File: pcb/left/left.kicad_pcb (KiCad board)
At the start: 2 copper layers, 27.9 x 72.4 mm, 21 parts, among them J1 Conn_01x07

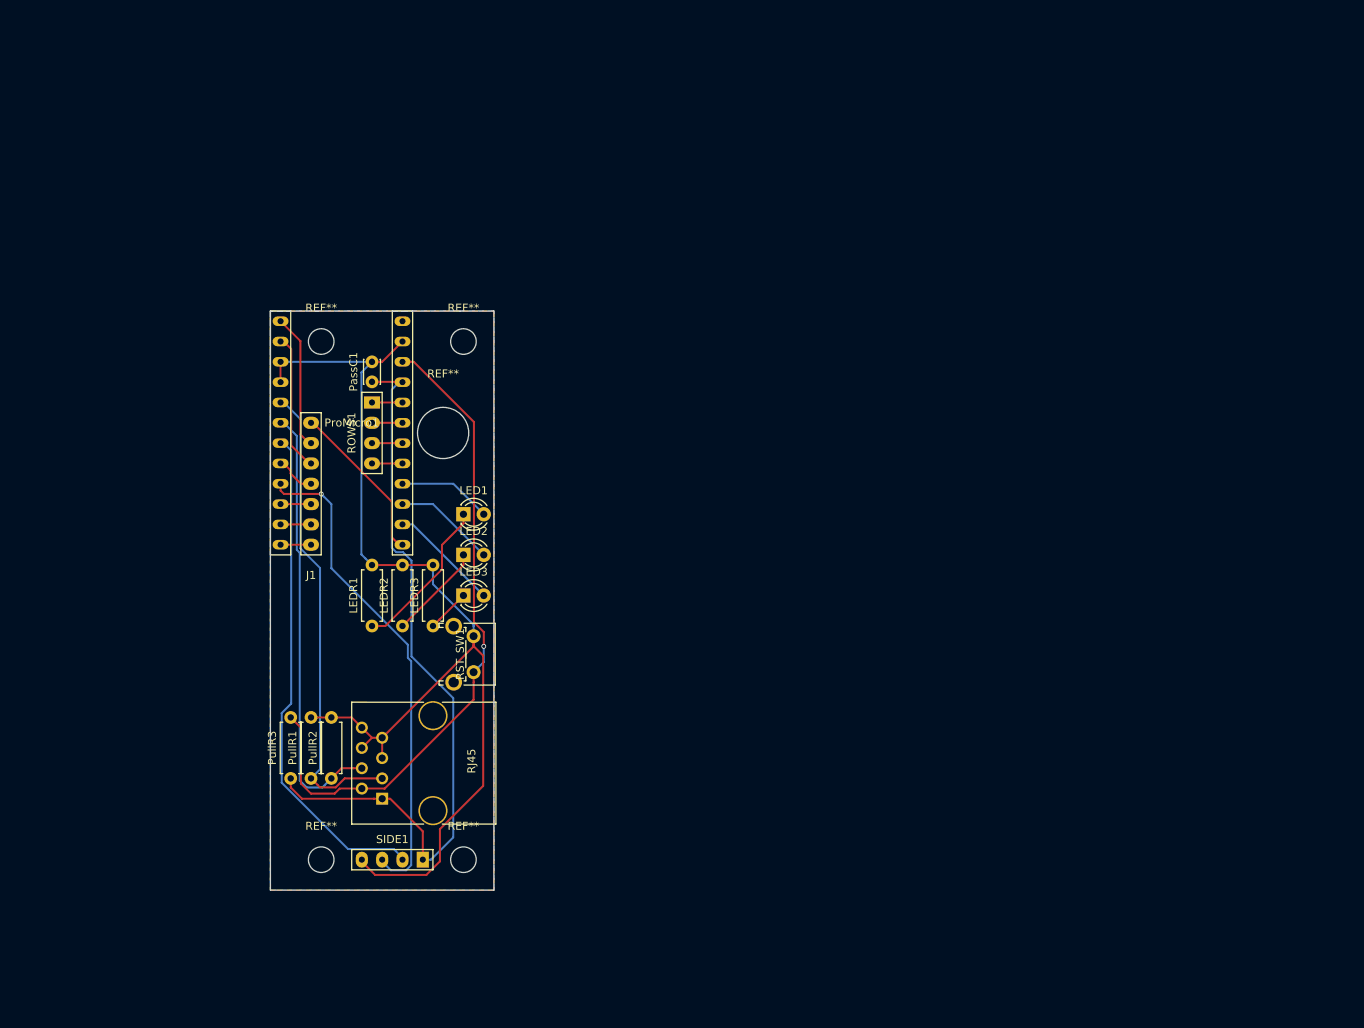
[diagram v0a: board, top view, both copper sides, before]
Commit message: left: large pcb
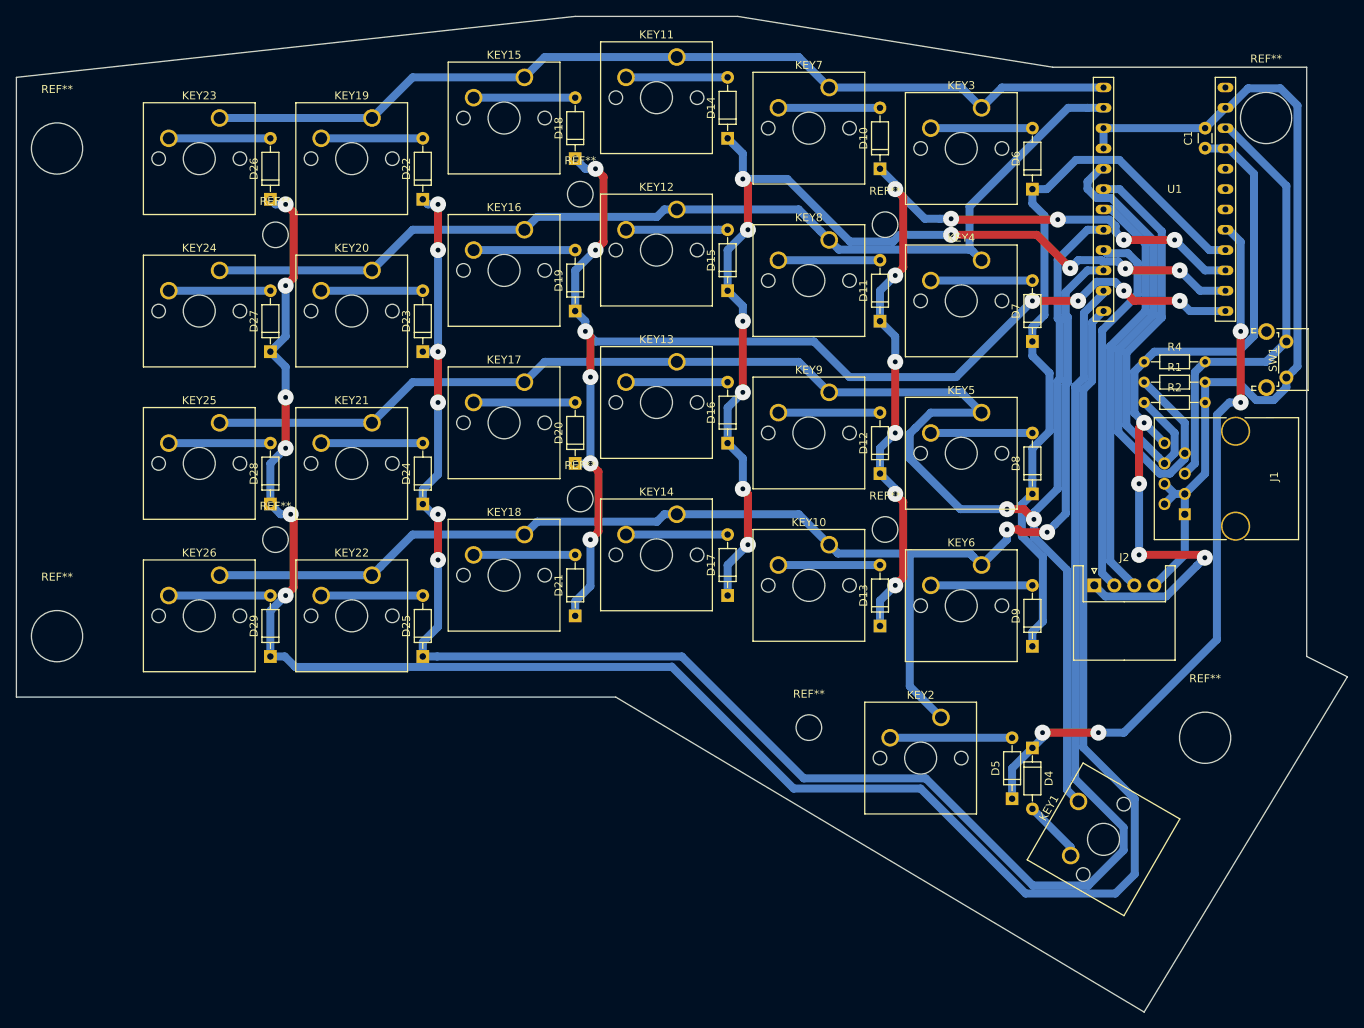
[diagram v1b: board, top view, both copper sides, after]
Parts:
- removed LED1: LED1, LEDs:LED_D3.0mm
- removed LED2: LED2, LEDs:LED_D3.0mm
- removed LED3: LED3, LEDs:LED_D3.0mm
- removed LEDR1: LED1_R, Resistors_THT:R_Axial_DIN0207_L6.3mm_D2.5mm_P7.62mm_Horizontal
- removed LEDR2: LED2_R, Resistors_THT:R_Axial_DIN0207_L6.3mm_D2.5mm_P7.62mm_Horizontal
- removed LEDR3: LED3_R, Resistors_THT:R_Axial_DIN0207_L6.3mm_D2.5mm_P7.62mm_Horizontal
- removed PassC1: PassC, Capacitors_THT:C_Disc_D3.0mm_W2.0mm_P2.50mm
- removed ProMicro1: Arduino_Pro_Micro, 4x6t2:Arduino_Pro_Micro
- removed PullR1, PullR2: I2C_PR, Resistors_THT:R_Axial_DIN0207_L6.3mm_D2.5mm_P7.62mm_Horizontal
- removed PullR3: RST_PR, Resistors_THT:R_Axial_DIN0207_L6.3mm_D2.5mm_P7.62mm_Horizontal
- removed the REF** at (55.9, 33.0)
- removed the REF** at (53.3, 44.5)
- removed the REF** at (55.9, 97.8)
- removed the REF** at (38.1, 33.0)
- removed the REF** at (38.1, 97.8)
- removed RJ45: RJ45-8pin, Connectors:RJ45_8
- removed ROWS1, SIDE1: Conn_01x04, 4x6t2:Wirepad_01x04
- removed RST_SW1: RST_Switch, Buttons_Switches_THT:SW_Tactile_SPST_Angled_PTS645Vx31-2LFS
- added C1: C, Capacitors_THT:C_Disc_D3.0mm_W1.6mm_P2.50mm, F.Cu at (148.6, 8.85)
- added D10: D, Diodes_THT:D_DO-35_SOD27_P7.62mm_Horizontal, F.Cu at (108.0, 11.4)
- added D11: D, Diodes_THT:D_DO-35_SOD27_P7.62mm_Horizontal, F.Cu at (108.0, 30.5)
- added D12: D, Diodes_THT:D_DO-35_SOD27_P7.62mm_Horizontal, F.Cu at (108.0, 49.5)
- added D13: D, Diodes_THT:D_DO-35_SOD27_P7.62mm_Horizontal, F.Cu at (108.0, 68.6)
- added D14: D, Diodes_THT:D_DO-35_SOD27_P7.62mm_Horizontal, F.Cu at (88.9, 7.62)
- added D15: D, Diodes_THT:D_DO-35_SOD27_P7.62mm_Horizontal, F.Cu at (88.9, 26.7)
- added D16: D, Diodes_THT:D_DO-35_SOD27_P7.62mm_Horizontal, F.Cu at (88.9, 45.7)
- added D17: D, Diodes_THT:D_DO-35_SOD27_P7.62mm_Horizontal, F.Cu at (88.9, 64.8)
- added D18: D, Diodes_THT:D_DO-35_SOD27_P7.62mm_Horizontal, F.Cu at (69.8, 10.2)
- added D19: D, Diodes_THT:D_DO-35_SOD27_P7.62mm_Horizontal, F.Cu at (69.8, 29.2)
- added D20: D, Diodes_THT:D_DO-35_SOD27_P7.62mm_Horizontal, F.Cu at (69.8, 48.3)
- added D21: D, Diodes_THT:D_DO-35_SOD27_P7.62mm_Horizontal, F.Cu at (69.8, 67.3)
- added D22: D, Diodes_THT:D_DO-35_SOD27_P7.62mm_Horizontal, F.Cu at (50.8, 15.2)
- added D23: D, Diodes_THT:D_DO-35_SOD27_P7.62mm_Horizontal, F.Cu at (50.8, 34.3)
- added D24: D, Diodes_THT:D_DO-35_SOD27_P7.62mm_Horizontal, F.Cu at (50.8, 53.3)
- added D25: D, Diodes_THT:D_DO-35_SOD27_P7.62mm_Horizontal, F.Cu at (50.8, 72.4)
- added D26: D, Diodes_THT:D_DO-35_SOD27_P7.62mm_Horizontal, F.Cu at (31.8, 15.2)
- added D27: D, Diodes_THT:D_DO-35_SOD27_P7.62mm_Horizontal, F.Cu at (31.8, 34.3)
- added D28: D, Diodes_THT:D_DO-35_SOD27_P7.62mm_Horizontal, F.Cu at (31.8, 53.3)
- added D29: D, Diodes_THT:D_DO-35_SOD27_P7.62mm_Horizontal, F.Cu at (31.8, 72.4)
- added D4: D, Diodes_THT:D_DO-35_SOD27_P7.62mm_Horizontal, F.Cu at (127.0, 83.8)
- added D5: D, Diodes_THT:D_DO-35_SOD27_P7.62mm_Horizontal, F.Cu at (124.5, 90.2)
- added D6: D, Diodes_THT:D_DO-35_SOD27_P7.62mm_Horizontal, F.Cu at (127.0, 14.0)
- added D7: D, Diodes_THT:D_DO-35_SOD27_P7.62mm_Horizontal, F.Cu at (127.0, 33.0)
- added D8: D, Diodes_THT:D_DO-35_SOD27_P7.62mm_Horizontal, F.Cu at (127.0, 52.1)
- added D9: D, Diodes_THT:D_DO-35_SOD27_P7.62mm_Horizontal, F.Cu at (127.0, 71.1)
- added J2: sidebutton, Connectors_JST:JST_XH_S04B-XH-A_04x2.50mm_Angled, F.Cu at (134.7, 63.5)
- added KEY1: KEY20, Buttons_Switches_Keyboard:SW_Cherry_MX1A_1.00u_PCB, F.Cu at (132.8, 90.5)
- added KEY10: KEY32, Buttons_Switches_Keyboard:SW_Cherry_MX1A_1.00u_PCB, F.Cu at (101.6, 58.4)
- added KEY11: KEY03, Buttons_Switches_Keyboard:SW_Cherry_MX1A_1.00u_PCB, F.Cu at (82.5, -2.54)
- added KEY12: KEY13, Buttons_Switches_Keyboard:SW_Cherry_MX1A_1.00u_PCB, F.Cu at (82.5, 16.5)
- added KEY13: KEY23, Buttons_Switches_Keyboard:SW_Cherry_MX1A_1.00u_PCB, F.Cu at (82.5, 35.6)
- added KEY14: KEY33, Buttons_Switches_Keyboard:SW_Cherry_MX1A_1.00u_PCB, F.Cu at (82.5, 54.6)
- added KEY15: KEY04, Buttons_Switches_Keyboard:SW_Cherry_MX1A_1.00u_PCB, F.Cu at (63.5, 0.00)
- added KEY16: KEY14, Buttons_Switches_Keyboard:SW_Cherry_MX1A_1.00u_PCB, F.Cu at (63.5, 19.1)
- added KEY17: KEY24, Buttons_Switches_Keyboard:SW_Cherry_MX1A_1.00u_PCB, F.Cu at (63.5, 38.1)
- added KEY18: KEY34, Buttons_Switches_Keyboard:SW_Cherry_MX1A_1.00u_PCB, F.Cu at (63.5, 57.1)
- added KEY19: KEY05, Buttons_Switches_Keyboard:SW_Cherry_MX1A_1.00u_PCB, F.Cu at (44.5, 5.08)
- added KEY2: KEY30, Buttons_Switches_Keyboard:SW_Cherry_MX1A_1.00u_PCB, F.Cu at (115.6, 80.0)
- added KEY20: KEY15, Buttons_Switches_Keyboard:SW_Cherry_MX1A_1.00u_PCB, F.Cu at (44.5, 24.1)
- added KEY21: KEY25, Buttons_Switches_Keyboard:SW_Cherry_MX1A_1.00u_PCB, F.Cu at (44.5, 43.2)
- added KEY22: KEY35, Buttons_Switches_Keyboard:SW_Cherry_MX1A_1.00u_PCB, F.Cu at (44.5, 62.2)
- added KEY23: KEY06, Buttons_Switches_Keyboard:SW_Cherry_MX1A_1.00u_PCB, F.Cu at (25.4, 5.08)
- added KEY24: KEY16, Buttons_Switches_Keyboard:SW_Cherry_MX1A_1.00u_PCB, F.Cu at (25.4, 24.1)
- added KEY25: KEY26, Buttons_Switches_Keyboard:SW_Cherry_MX1A_1.00u_PCB, F.Cu at (25.4, 43.2)
- added KEY26: KE36, Buttons_Switches_Keyboard:SW_Cherry_MX1A_1.00u_PCB, F.Cu at (25.4, 62.2)
- added KEY3: KEY01, Buttons_Switches_Keyboard:SW_Cherry_MX1A_1.00u_PCB, F.Cu at (120.7, 3.81)
- added KEY4: KEY11, Buttons_Switches_Keyboard:SW_Cherry_MX1A_1.00u_PCB, F.Cu at (120.7, 22.9)
- added KEY5: KEY21, Buttons_Switches_Keyboard:SW_Cherry_MX1A_1.00u_PCB, F.Cu at (120.7, 41.9)
- added KEY6: KEY31, Buttons_Switches_Keyboard:SW_Cherry_MX1A_1.00u_PCB, F.Cu at (120.7, 61.0)
- added KEY7: KEY02, Buttons_Switches_Keyboard:SW_Cherry_MX1A_1.00u_PCB, F.Cu at (101.6, 1.27)
- added KEY8: KEY12, Buttons_Switches_Keyboard:SW_Cherry_MX1A_1.00u_PCB, F.Cu at (101.6, 20.3)
- added KEY9: KEY22, Buttons_Switches_Keyboard:SW_Cherry_MX1A_1.00u_PCB, F.Cu at (101.6, 39.4)
- added R1: 10kΩ, Resistors_THT:R_Axial_DIN0204_L3.6mm_D1.6mm_P7.62mm_Horizontal, F.Cu at (141.0, 38.1)
- added R2: 10kΩ, Resistors_THT:R_Axial_DIN0204_L3.6mm_D1.6mm_P7.62mm_Horizontal, F.Cu at (141.0, 40.6)
- added R4: R, Resistors_THT:R_Axial_DIN0204_L3.6mm_D1.6mm_P7.62mm_Horizontal, F.Cu at (141.0, 35.6)
- added REF**: MountingHole_3.2mm_M3, Mounting_Holes:MountingHole_3.2mm_M3, F.Cu at (70.5, 14.6)
- added REF**: MountingHole_6.4mm_M6, Mounting_Holes:MountingHole_6.4mm_M6, F.Cu at (156.2, 5.08)
- added REF**: MountingHole_6.4mm_M6, Mounting_Holes:MountingHole_6.4mm_M6, F.Cu at (148.6, 82.5)
- added REF**: MountingHole_3.2mm_M3, Mounting_Holes:MountingHole_3.2mm_M3, F.Cu at (70.5, 52.7)
- added REF**: MountingHole_3.2mm_M3, Mounting_Holes:MountingHole_3.2mm_M3, F.Cu at (32.4, 19.7)
- added REF**: MountingHole_3.2mm_M3, Mounting_Holes:MountingHole_3.2mm_M3, F.Cu at (32.4, 57.8)
- added REF**: MountingHole_3.2mm_M3, Mounting_Holes:MountingHole_3.2mm_M3, F.Cu at (108.6, 18.4)
- added REF**: MountingHole_3.2mm_M3, Mounting_Holes:MountingHole_3.2mm_M3, F.Cu at (108.6, 56.5)
- added REF**: MountingHole_3.2mm_M3, Mounting_Holes:MountingHole_3.2mm_M3, F.Cu at (99.1, 81.3)
- added REF**: MountingHole_6.4mm_M6, Mounting_Holes:MountingHole_6.4mm_M6, F.Cu at (5.08, 8.89)
- added REF**: MountingHole_6.4mm_M6, Mounting_Holes:MountingHole_6.4mm_M6, F.Cu at (5.08, 69.8)
- added SW1: RESET_SW, Buttons_Switches_THT:SW_Tactile_SPST_Angled_PTS645Vx31-2LFS, F.Cu at (158.8, 33.0)
- added U1: Arduino_Pro_Micro, 4x6t2:Arduino_Pro_Micro, F.Cu at (144.8, 15.2)
- J1: value Conn_01x07 -> RJ45-8pin; footprint 4x6t2:Wirepad_01x07 -> Connectors:RJ45_8
- moved J1 109.2 mm to (146.1, 54.6), turned to 90 degrees
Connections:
- J1 pad 1: /Thumb_key -> GND
- J1 pad 2: /COL0 -> GND
- J1 pad 3: /COL1 -> GND
- J1 pad 4: /COL2 -> GND
- J1 pad 5: /COL3 -> /RST
- J1 pad 6: /COL4 -> /SCL
- J1 pad 7: /COL5 -> /SDA
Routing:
- net /COL6: track 0.00 -> 260.5 mm, vias 0 -> 6
- net /COL5: track 3.81 -> 238.5 mm, vias 0 -> 6
- net /ROW2: track 3.81 -> 211.6 mm, vias 0 -> 2
- net /ROW4: track 0.00 -> 171.1 mm, vias 0 -> 2
- net /COL4: track 3.81 -> 154.0 mm, vias 0 -> 10
- net /COL3: track 3.81 -> 130.6 mm, vias 0 -> 10
- net /ROW1: track 3.81 -> 128.3 mm
- net /ROW0: track 3.81 -> 117.3 mm
- net /COL2: track 5.10 -> 109.4 mm, vias 0 -> 10
- net /COL1: track 17.2 -> 92.7 mm
- net /COL0: track 17.0 -> 90.8 mm, vias 0 -> 4
- net GND: track 137.9 -> 110.2 mm
- net /RST: track 83.6 -> 56.3 mm, vias 1 -> 0
- net /Thumb_key: track 20.3 -> 0.00 mm
- net Net-(LED1-Pad1): track 19.7 -> 0.00 mm
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- removed copper zone on B.Cu, net GND
- removed copper zone on F.Cu, net GND
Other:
- board size 27.9 x 72.4 mm -> 166.4 x 124.5 mm
- net class Default: clearance 0.203 -> 0.01; trace_width 0.25 -> 1; via_dia 0.6 -> 2; via_drill 0.4 -> 0.6
- rule trace_clearance: 0.203 -> 0.01
- rule trace_min: 0.203 -> 0.01
- rule via_min_drill: 0.3 -> 0.5
- rule via_min_size: 0.4 -> 1.27
